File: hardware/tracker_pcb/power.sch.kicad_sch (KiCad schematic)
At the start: 20 parts, among them U3 TPS62933FDRLR, U4 TPS2117DRLR, U5 TLV1117LV33DCYR

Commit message: ss changes
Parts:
- CR1: LCSC (none) -> C3759778
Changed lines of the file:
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@@
+			)
+		)
+		(property "LCSC" "C3759778"
+			(at 79.375 74.93 0)
+			(effects
+				(font
+					(size 1.27 1.27)
+				)
+				(hide yes)
 			)
 		)

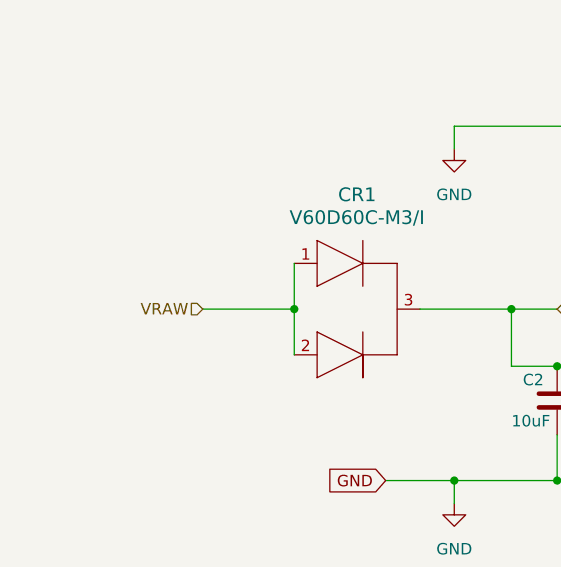
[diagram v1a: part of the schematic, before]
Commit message: Add fuseholder
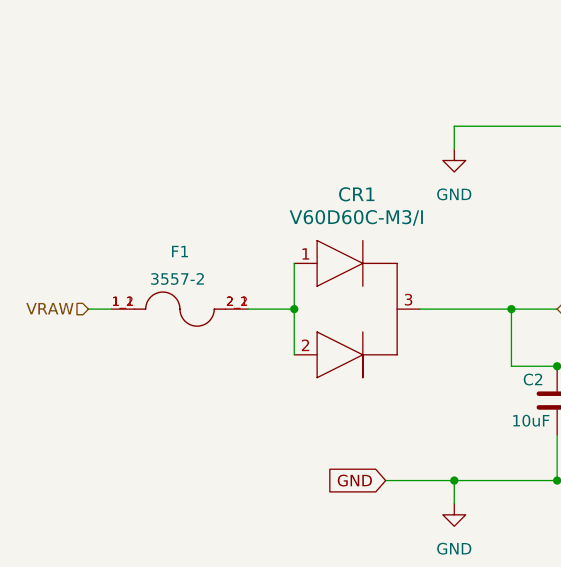
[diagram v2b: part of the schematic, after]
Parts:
- added F1: 3557-2, footprint:FUSE_3557-2, symbol symbol:3557-2
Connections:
- net VRAW: now also F1.1_1, F1.1_2; no longer CR1.1, CR1.2
- new net: CR1.1, CR1.2, F1.2_1, F1.2_2
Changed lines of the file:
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@@
 	(wire
 		(pts
-			(xy 62.23 87.63) (xy 72.39 87.63)
+			(xy 49.53 87.63) (xy 52.07 87.63)
 		)
 		(stroke
@@
 		(pts
 			(xy 215.9 46.99) (xy 204.47 46.99)
+		)
+		(stroke
+			(width 0)
+			(type default)
+		)
+	)
+	(wire
+		(pts
+			(xy 67.31 87.63) (xy 72.39 87.63)
 		)
 		(stroke
@@
 	(hierarchical_label "VRAW"
 		(shape input)
-		(at 62.23 87.63 180)
+		(at 49.53 87.63 180)
 		(effects
 			(font
@@
 					(unit 1)
 				)
+			)
+		)
+	)
+	(symbol
+		(lib_id "symbol:3557-2")
+		(at 59.69 87.63 0)
+		(unit 1)
+		(exclude_from_sim no)
+		(in_bom yes)
+		(on_board yes)
+		(dnp no)
+		(property "Reference" "F1"
+			(at 59.69 81.28 0)
+			(effects
+				(font
+					(size 1.27 1.27)
+				)
+			)
+		)
+		(property "Value" "3557-2"
+			(at 59.436 84.328 0)
+			(effects
+				(font
+					(size 1.27 1.27)
+				)
+			)
+		)
+		(property "Footprint" "footprint:FUSE_3557-2"
+			(at 59.69 87.63 0)
+			(effects
+				(font
+					(size 1.27 1.27)
+				)
+				(justify bottom)
+				(hide yes)
+			)
+		)
+		(property "Datasheet" ""
+			(at 59.69 87.63 0)
+			(effects
+				(font
+					(size 1.27 1.27)
+				)
+				(hide yes)
+			)
+		)
+		(property "Description" ""
+			(at 59.69 87.63 0)
+			(effects
+				(font
+					(size 1.27 1.27)
+				)
+				(hide yes)
+			)
+		)
+		(property "PARTREV" "D"
+			(at 59.69 87.63 0)
+			(effects
+				(font
+					(size 1.27 1.27)
+				)
+				(justify bottom)
+				(hide yes)
+			)
+		)
+		(property "STANDARD" "Manufacturer Recommendation"
+			(at 59.69 87.63 0)
+			(effects
+				(font
+					(size 1.27 1.27)
+				)
+				(justify bottom)
+				(hide yes)
+			)
+		)
+		(property "SNAPEDA_PN" "3557-2"
+			(at 59.69 87.63 0)
+			(effects
+				(font
+					(size 1.27 1.27)
+				)
+				(justify bottom)
+				(hide yes)
+			)
+		)
+		(property "MAXIMUM_PACKAGE_HEIGHT" "7.37mm"
+			(at 59.69 87.63 0)
+			(effects
+				(font
+					(size 1.27 1.27)
+				)
+				(justify bottom)
+				(hide yes)
+			)
+		)
+		(property "MANUFACTURER" "Keystone"
+			(at 59.69 87.63 0)
+			(effects
+				(font
+					(size 1.27 1.27)
+				)
+				(justify bottom)
+				(hide yes)
+			)
+		)
+		(pin "1_2"
+		)
+		(pin "2_1"
+		)
+		(pin "1_1"
+		)
+		(pin "2_2"
+		)
+		(instances
+			(project ""
+				(path "/6aaa9514-f94e-4843-90d0-16960e4e49cb/4c324161-c4da-41f3-8af5-33f4b9a0442d"
+					(reference "F1")
+					(unit 1)
+				)
